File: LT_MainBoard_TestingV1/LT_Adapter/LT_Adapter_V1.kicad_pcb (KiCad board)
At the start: 2 copper layers, 68 x 65.5 mm, 9 parts, among them CN1 NUCLEO-L432KC, U1 XBP9B-DPST-001

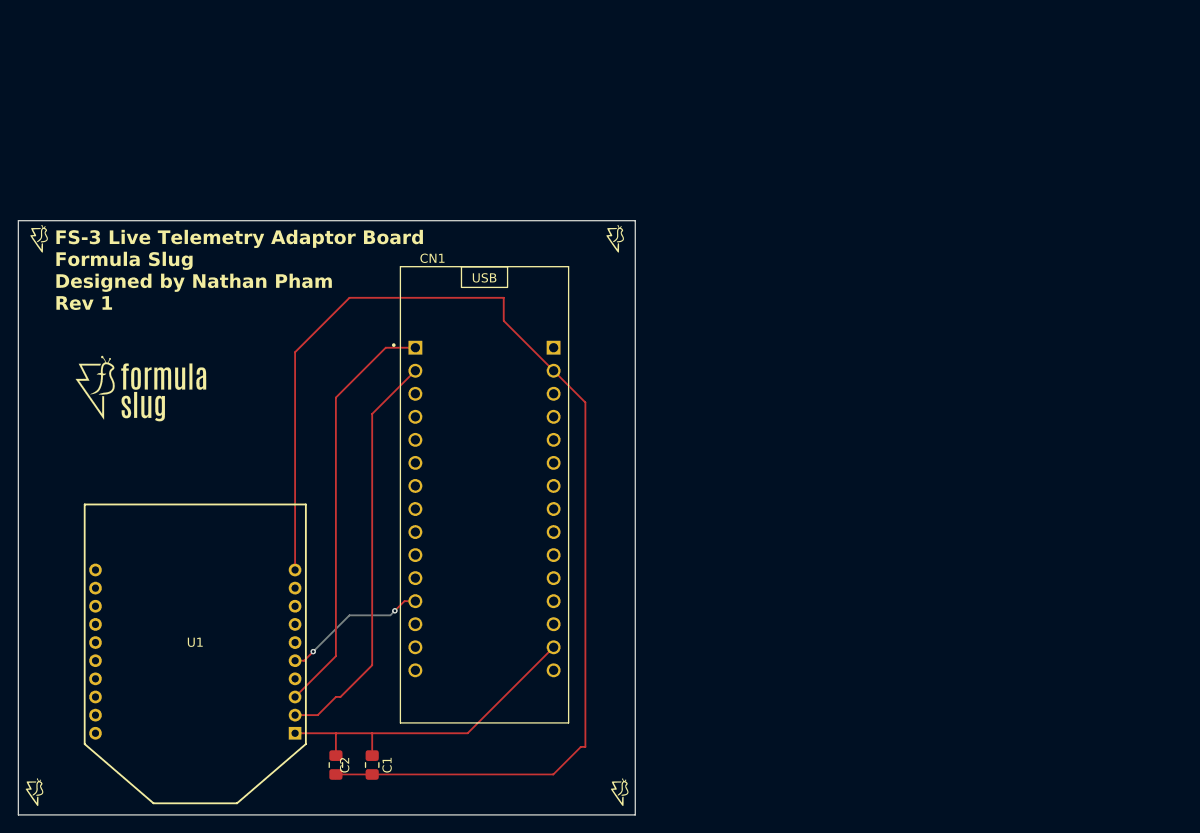
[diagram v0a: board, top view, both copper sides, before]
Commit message: Adapter Board
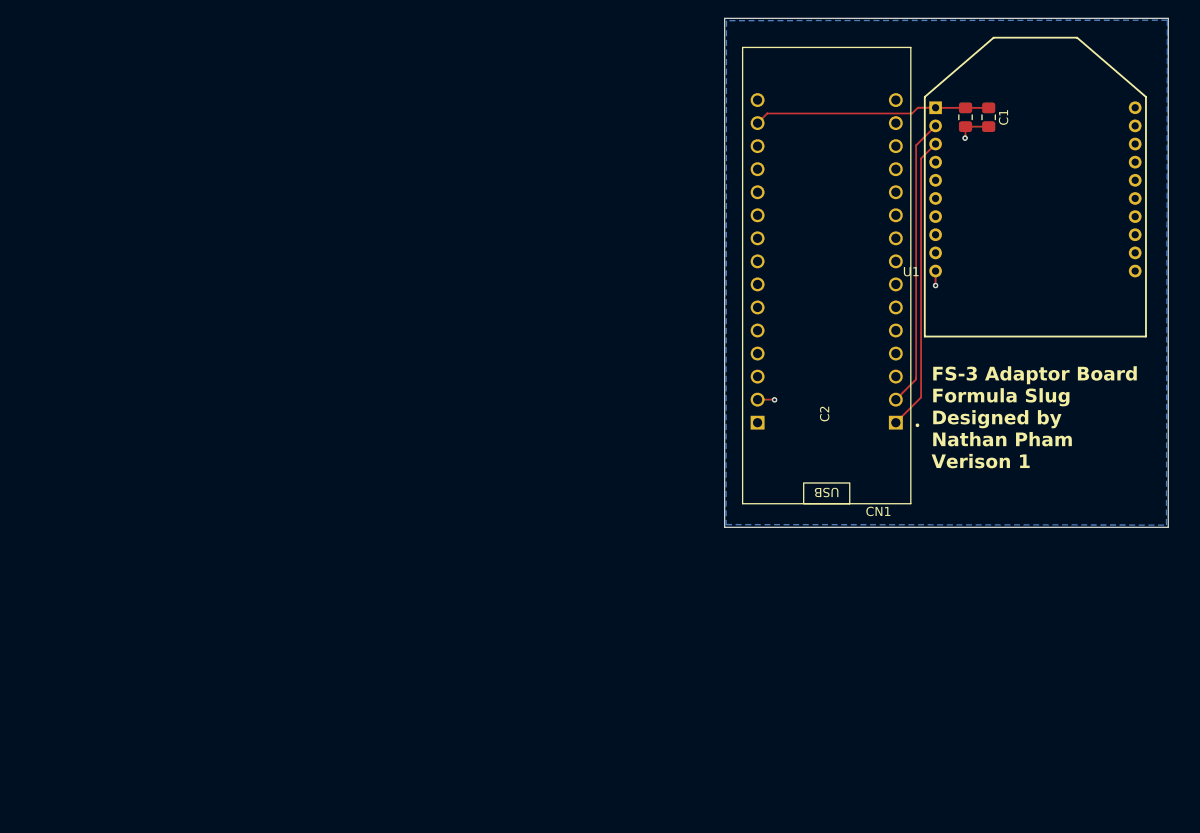
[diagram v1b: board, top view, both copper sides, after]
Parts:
- removed G*** (x4): LOGO, FS_3_Global_Footprint_Library:FORMULA SLUG
- removed G***: LOGO, FSFootprints:fs_logo_full_2400
- moved U1 105.9 mm to (148.1, 61.3), turned to 0 degrees
- moved C2 99.6 mm to (140.4, 53.6)
- moved C1 98.6 mm to (142.9, 53.6)
- moved CN1 44.8 mm to (125.1, 71.0), turned to 180 degrees
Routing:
- net GND: track 131.9 -> 7.31 mm, vias 0 -> 3
- net /RADIO_RESET: track 16.0 -> 0.00 mm, vias 2 -> 0
- net /RADIO_IN: track 45.9 -> 32.5 mm
- net /RADIO_OUT: track 45.2 -> 32.0 mm
- net +3V3: track 37.4 -> 26.2 mm
- added copper zone on B.Cu, net GND
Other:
- board size 68 x 65.5 mm -> 48.9 x 56.1 mm
- board text added: "FS-3 Adaptor Board Formula Slug Designed by Nathan Pham Verison 1"
- board text removed: "FS-3 Live Telemetry Adaptor Board Formula Slug Designed by Nathan Pham Rev 1"
